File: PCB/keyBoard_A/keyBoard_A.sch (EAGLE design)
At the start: 262 parts, among them J1 J, J10 J, J11 J, J12 J, J13 J, J14 J, J15 J, J16 J, J17 J, J18 J, J19 J, J2 J, J20 J, J21 J, J22 J, J23 J, J24 J, J25 J, J26 J, J27 J, J28 J, J29 J, J3 J, J30 J, J31 J, J32 J, J33 J, J34 J, J35 J, J36 J, J37 J, J38 J, J39 J, J4 J, J40 J, J41 J, J42 J, J43 J, J44 J, J45 J, J46 J, J47 J, J48 J, J49 J, J5 J, J50 J, J51 J, J52 J, J53 J, J54 J, J55 J, J56 J, J57 J, J6 J, J7 J, J8 J, J9 J

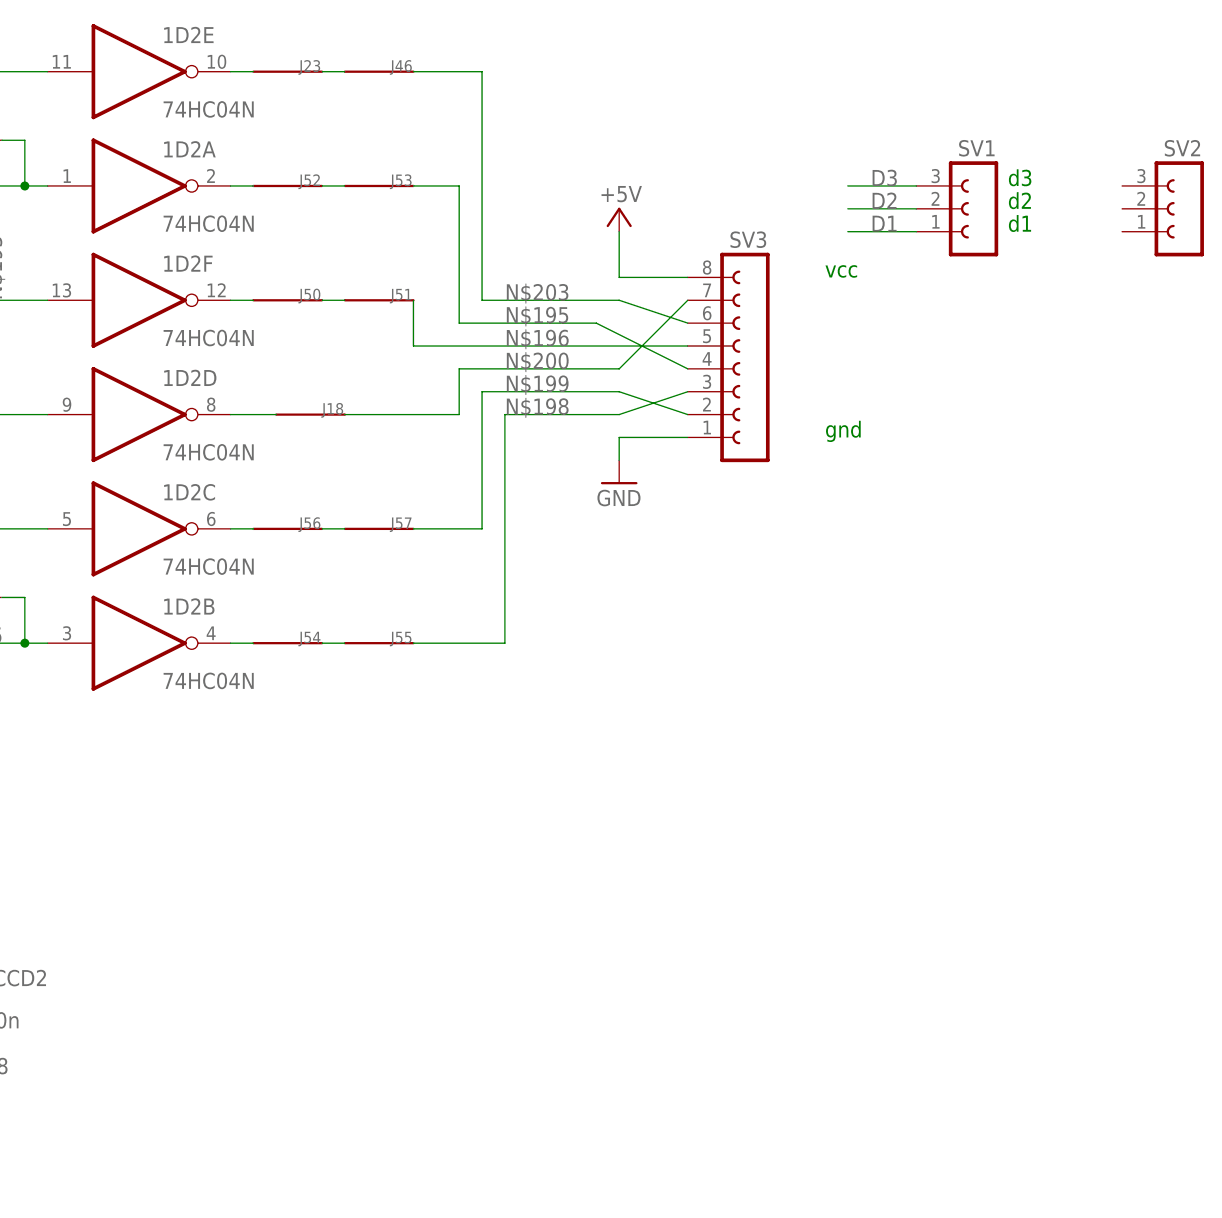
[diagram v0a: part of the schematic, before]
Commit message: pcb a r
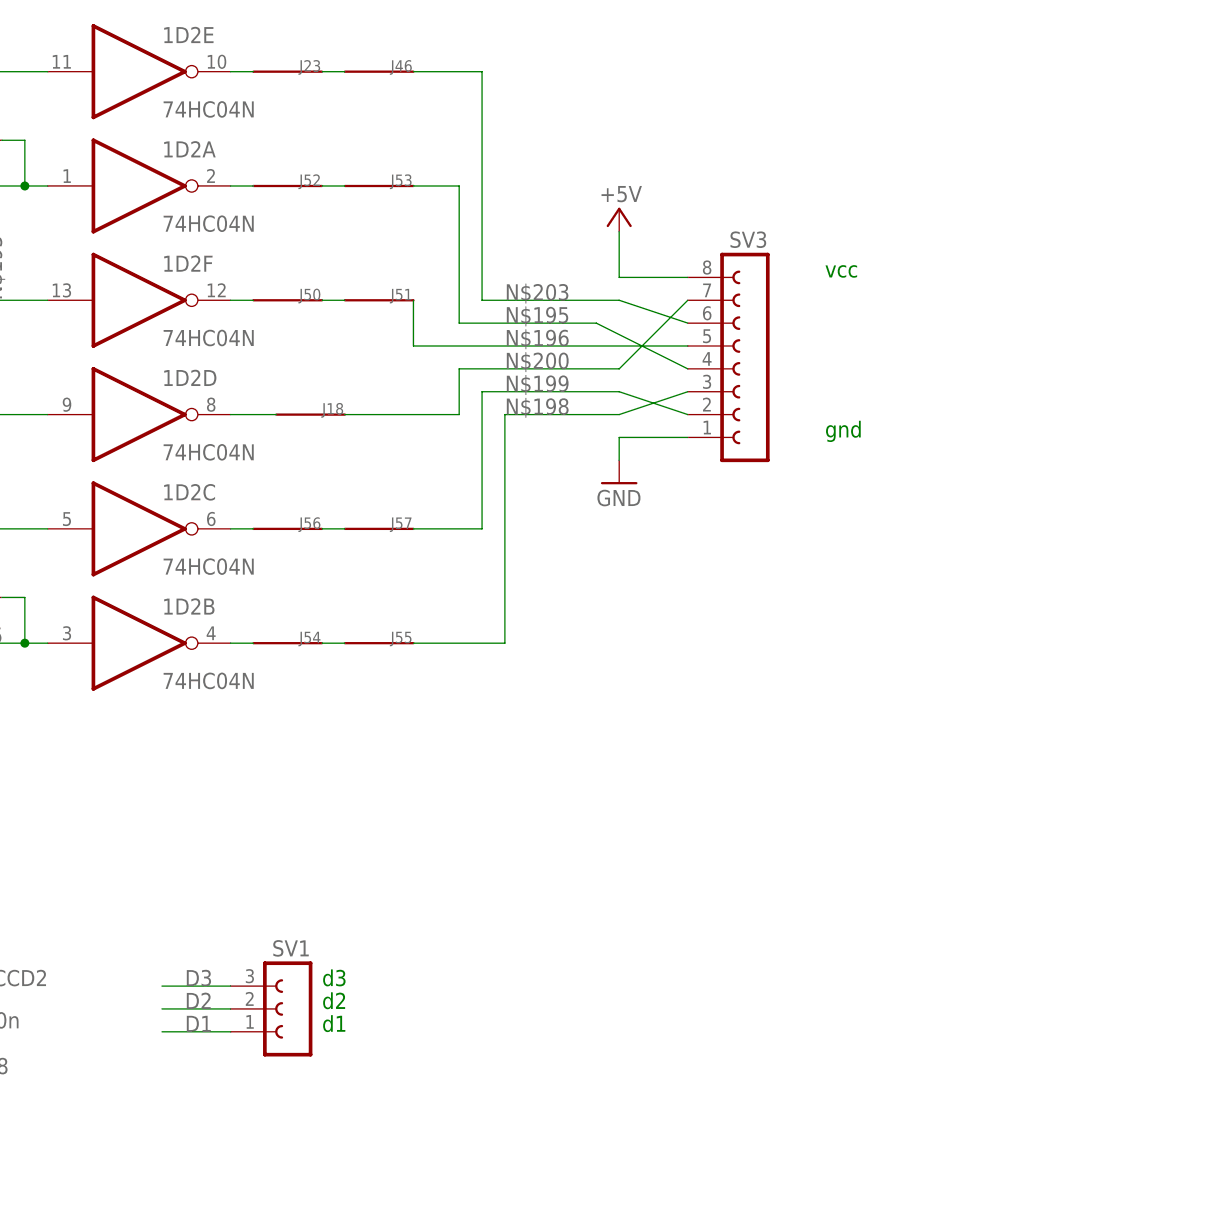
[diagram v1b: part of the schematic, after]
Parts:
- removed SV2: (no value), detali_main:FE03-1
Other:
- moved on the sheet: SV1
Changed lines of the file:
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@@
 <part name="J49" library="detali_main" deviceset="J" device=""/>
 <part name="R10" library="rd" deviceset="RD" device="" value="10k"/>
-<part name="SV2" library="detali_main" deviceset="FE03-1" device="">
-<attribute name="MF" value=""/>
-<attribute name="MPN" value=""/>
-<attribute name="OC_FARNELL" value="unknown"/>
-<attribute name="OC_NEWARK" value="unknown"/>
-</part>
 <part name="J18" library="detali_main" deviceset="J" device=""/>
 <part name="R100" library="rd" deviceset="RD" device="" value="10k"/>
@@
 <description>KB_A</description>
 <plain>
-<text x="398.78" y="317.5" size="1.778" layer="91">d1</text>
+<text x="322.58" y="228.6" size="1.778" layer="91">d1</text>
 <text x="378.46" y="312.42" size="1.778" layer="91">vcc</text>
-<text x="398.78" y="320.04" size="1.778" layer="91">d2</text>
-<text x="398.78" y="322.58" size="1.778" layer="91">d3</text>
+<text x="322.58" y="231.14" size="1.778" layer="91">d2</text>
+<text x="322.58" y="233.68" size="1.778" layer="91">d3</text>
 <text x="378.46" y="294.64" size="1.778" layer="91">gnd</text>
 <text x="40.64" y="304.8" size="5.08" layer="91">LEFT KB</text>
@@
 <instance part="JB88" gate="1" x="114.3" y="269.24"/>
 <instance part="D88" gate="G$1" x="104.14" y="269.24"/>
-<instance part="SV1" gate="G$1" x="396.24" y="322.58" rot="MR0"/>
+<instance part="SV1" gate="G$1" x="320.04" y="233.68" rot="MR0"/>
 <instance part="SV3" gate="G$1" x="370.84" y="302.26" rot="MR0"/>
 <instance part="J47" gate="G$1" x="45.72" y="104.14"/>
@@
 <attribute name="VALUE" x="252.73" y="327.66" size="1.778" layer="95"/>
 </instance>
-<instance part="SV2" gate="G$1" x="419.1" y="322.58" rot="MR0"/>
 <instance part="J18" gate="G$1" x="320.04" y="297.18" smashed="yes">
 <attribute name="NAME" x="322.58" y="297.18" size="1.27" layer="95"/>
@@
 <segment>
 <pinref part="SV1" gate="G$1" pin="3"/>
-<wire x1="388.62" y1="322.58" x2="381" y2="322.58" width="0.1524" layer="91"/>
-<label x="383.54" y="322.58" size="1.778" layer="95"/>
+<wire x1="312.42" y1="233.68" x2="304.8" y2="233.68" width="0.1524" layer="91"/>
+<label x="307.34" y="233.68" size="1.778" layer="95"/>
 </segment>
 </net>
@@
 <segment>
 <pinref part="SV1" gate="G$1" pin="2"/>
-<wire x1="381" y1="320.04" x2="388.62" y2="320.04" width="0.1524" layer="91"/>
-<label x="383.54" y="320.04" size="1.778" layer="95"/>
+<wire x1="304.8" y1="231.14" x2="312.42" y2="231.14" width="0.1524" layer="91"/>
+<label x="307.34" y="231.14" size="1.778" layer="95"/>
 </segment>
 </net>
@@
 <segment>
 <pinref part="SV1" gate="G$1" pin="1"/>
-<wire x1="388.62" y1="317.5" x2="381" y2="317.5" width="0.1524" layer="91"/>
-<label x="383.54" y="317.5" size="1.778" layer="95"/>
-</segment>
-</net>
+<wire x1="312.42" y1="228.6" x2="304.8" y2="228.6" width="0.1524" layer="91"/>
+<label x="307.34" y="228.6" size="1.778" layer="95"/>
+</segment>
+</net>

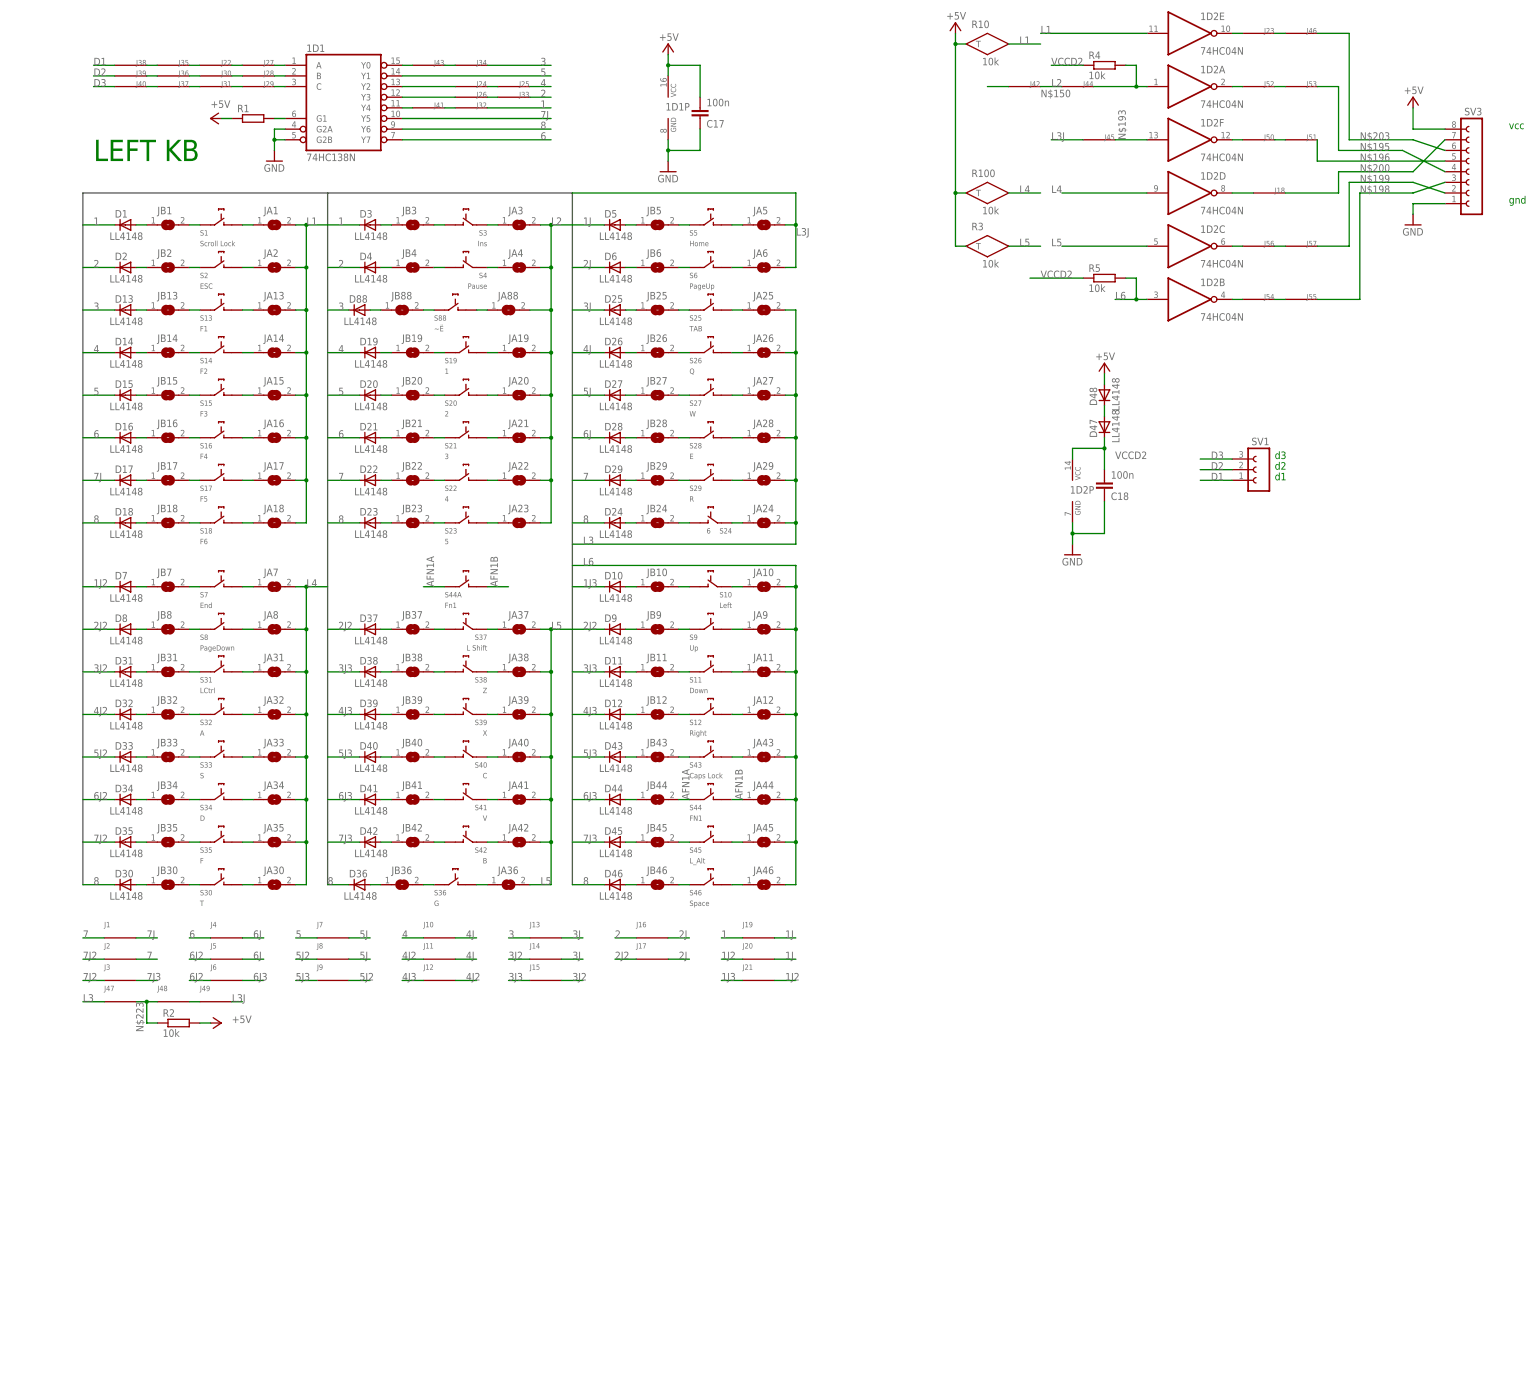
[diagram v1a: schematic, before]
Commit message: pcb a
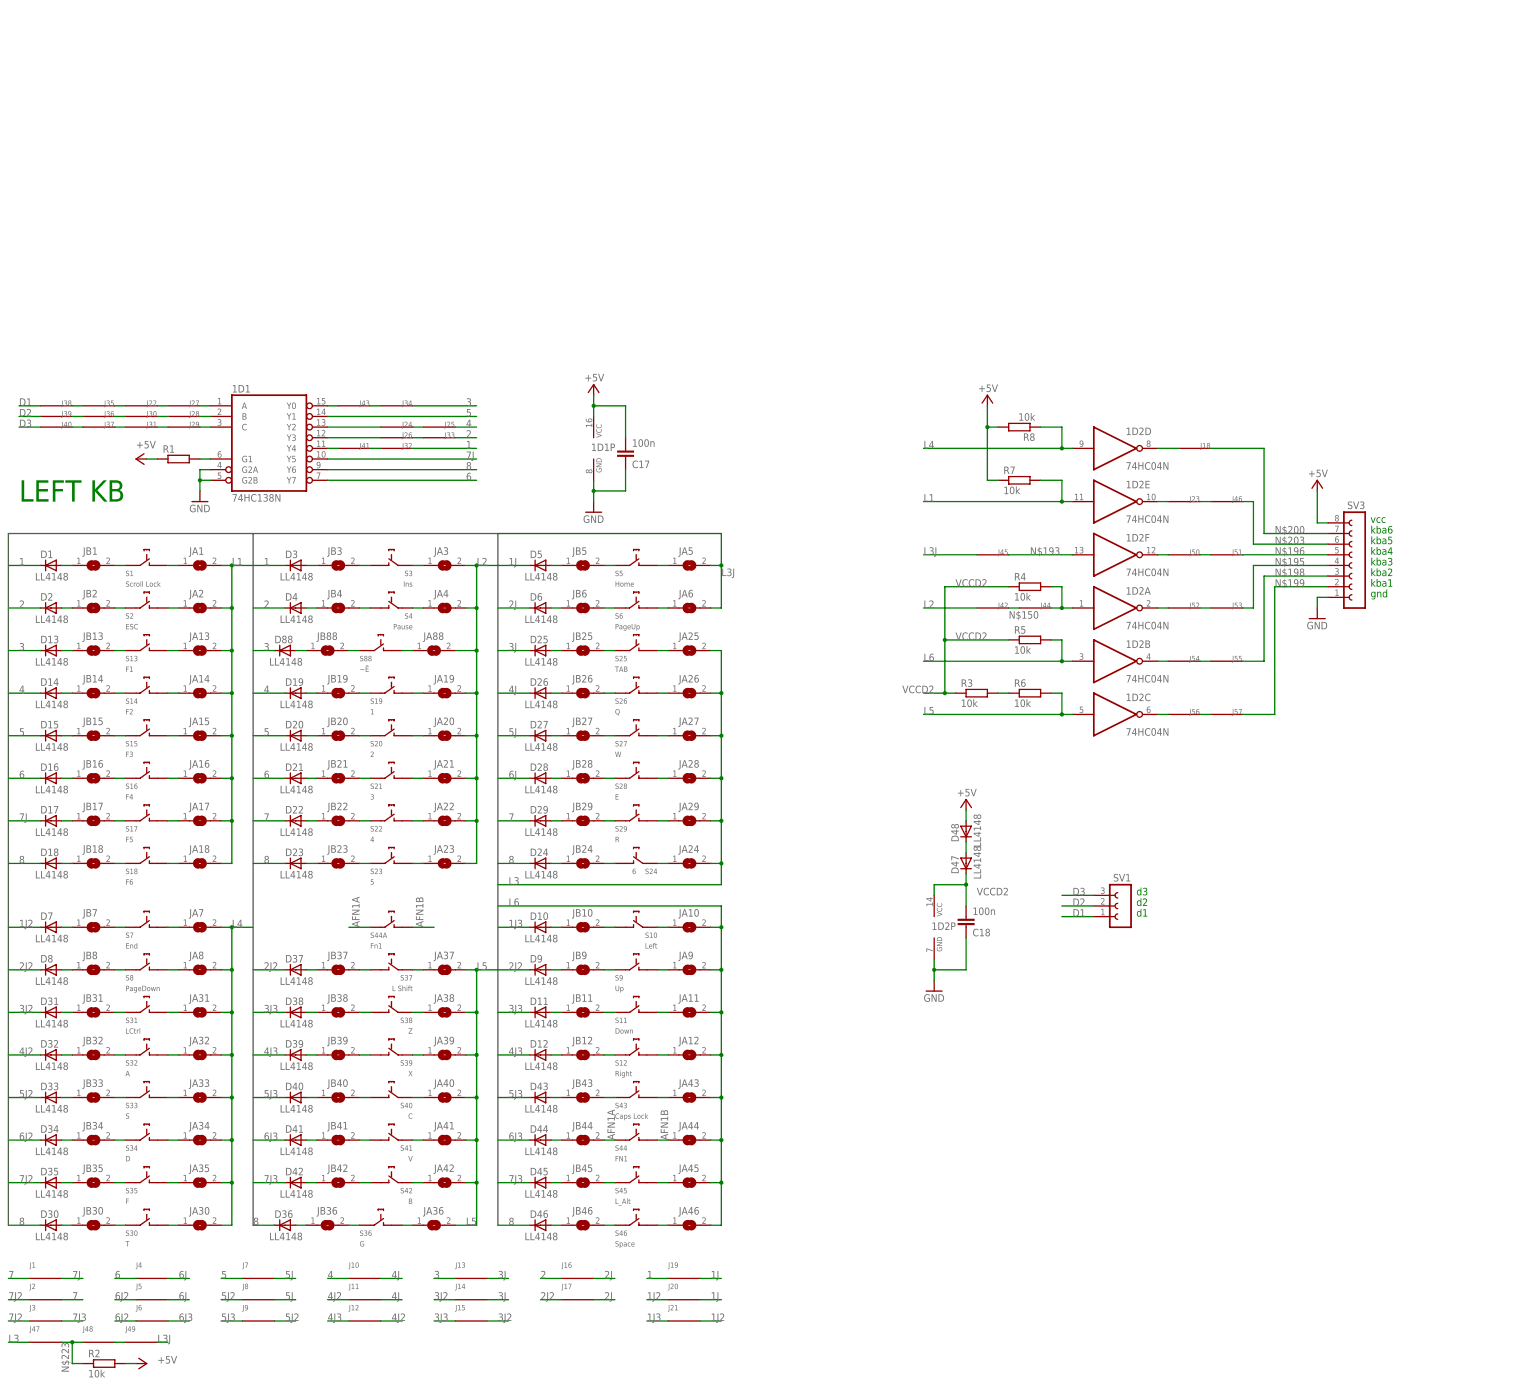
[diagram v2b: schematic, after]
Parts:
- removed R10, R100: 10k, rd:RD
- added R6, R7: 10k, rcl:R-EU_R1206W
- added R8: 10k, rcl:R-EU_R0805
- R3: device rd:RD -> rcl:R-EU_R1206W
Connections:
- new net N$238: R3.2, R6.1
- net +5V: now also R7.1, R8.2; no longer R10.T, R100.T, R3.T
- net L1: now also R7.2; no longer R10.B
- net L4: now also R8.1; no longer R100.B
- net L5: now also R6.2; no longer R3.B
- net VCCD2: now also R3.1
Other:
- note added: "kba1"
- note added: "kba2"
- note added: "kba3"
- note added: "kba4"
- note added: "kba5"
- note added: "kba6"
- moved on the sheet: 1D1, 1D1P, 1D2A, 1D2B, 1D2C, 1D2D, 1D2E, 1D2F, 1D2P, C17, C18, D1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
